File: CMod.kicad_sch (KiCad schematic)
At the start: 2 parts

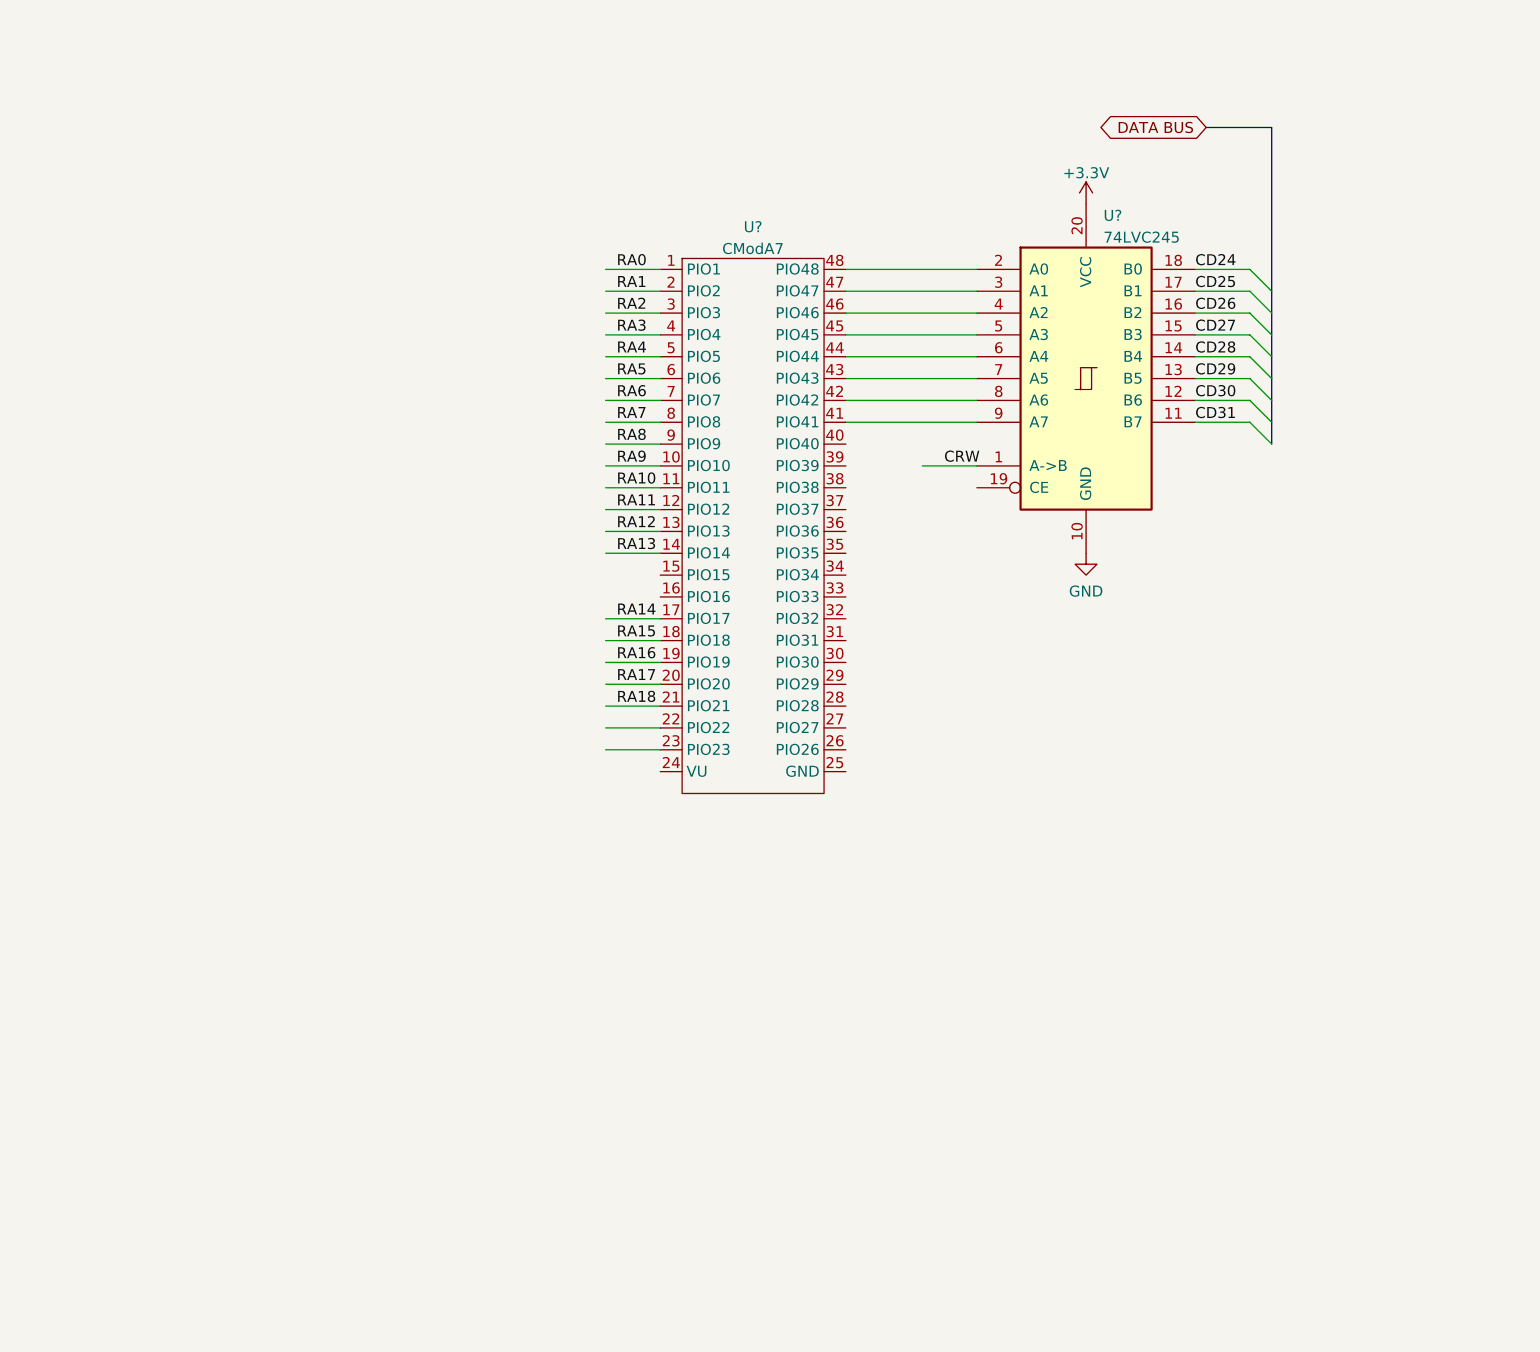
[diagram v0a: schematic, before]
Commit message: ISA68030 - update
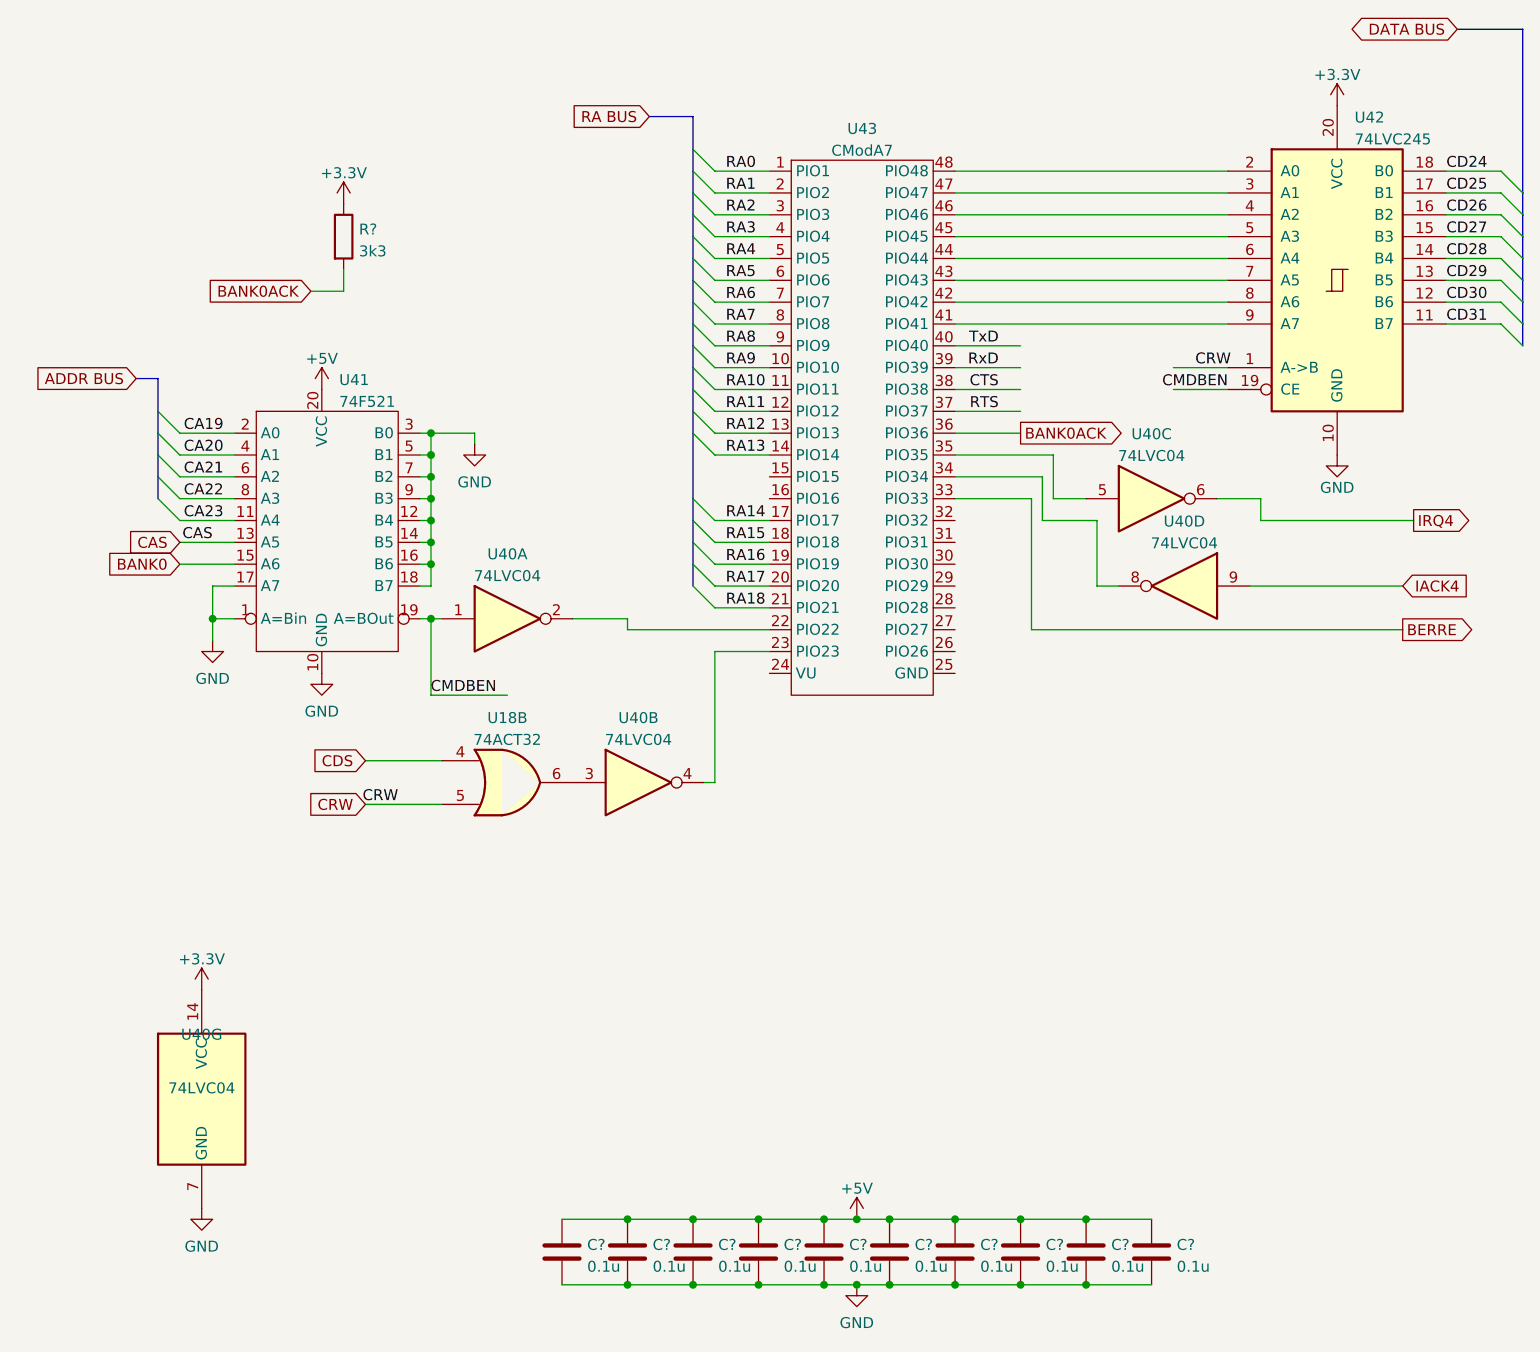
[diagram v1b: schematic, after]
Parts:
- added C? (x10): 0.1u, symbol Device:C
- added R?: 3k3, symbol Device:R
- added U18: 74ACT32, symbol 74xx:74LS32
- added U40: 74LVC04, symbol 74xx:74LS04
- added U41: 74F521, symbol MyLib:74F521
- gave numbers to parts that had none: 2
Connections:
- net +3.3V: now also R?.1, U40.14 (VCC)
- net CRW: now also U18.5
- net GND: now also C?.2, C?.2, C?.2, C?.2, C?.2, C?.2, C?.2, C?.2, C?.2, C?.2, U40.7 (GND), U41.1 (A=Bin), U41.10 (GND), U41.12 (B4), U41.14 (B5), U41.16 (B6), U41.17 (A7), U41.18 (B7), U41.3 (B0), U41.5 (B1), U41.7 (B2), U41.9 (B3)
- net CMDBEN: now reaches U42.19 (CE)
- net CMDBEN: now also U40.1, U41.19 (A=BOut)
- net at U43.22 (PIO22): now also U40.2
- net at U43.23 (PIO23): now also U40.4
- net BERRE: now reaches U43.33 (PIO33)
- net at U43.34 (PIO34): now also U40.8
- net at U43.35 (PIO35): now also U40.5
- net BANK0ACK: now reaches U43.36 (PIO36)
- net BANK0ACK: now also R?.2
- net RTS: now reaches U43.37 (PIO37)
- net CTS: now reaches U43.38 (PIO38)
- net RxD: now reaches U43.39 (PIO39)
- net TxD: now reaches U43.40 (PIO40)
- new net: U18.6, U40.3
- new net +5V: C?.1, C?.1, C?.1, C?.1, C?.1, C?.1, C?.1, C?.1, C?.1, C?.1, U41.20 (VCC)
- new net BANK0: U41.15 (A6)
- new net CA19: U41.2 (A0)
- new net CA20: U41.4 (A1)
- new net CA21: U41.6 (A2)
- new net CA22: U41.8 (A3)
- new net CA23: U41.11 (A4)
- new net CAS: U41.13 (A5)
- new net CDS: U18.4
- new net IACK4: U40.9
- new net IRQ4: U40.6
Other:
- company: (none) -> Finitron
- title: (none) -> ISA68030 Boot ROM, Keyboard, Mouse
- moved on the sheet: U42, U43
